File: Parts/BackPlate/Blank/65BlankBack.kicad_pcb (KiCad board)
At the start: 2 copper layers, 172.9 x 20 mm, 3 parts

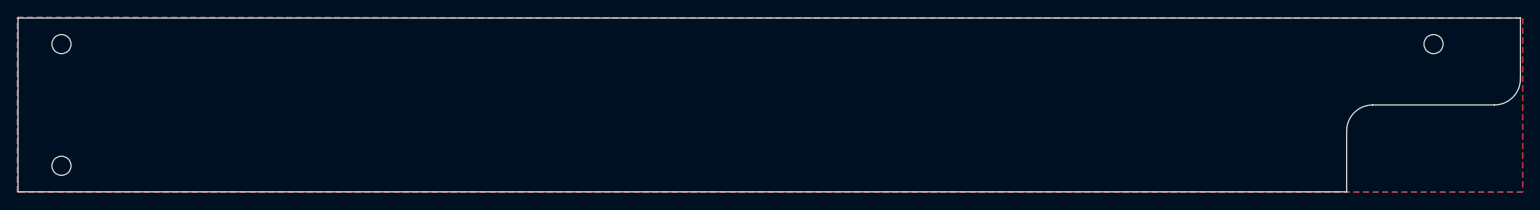
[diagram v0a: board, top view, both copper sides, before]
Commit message: 寸法更新とか
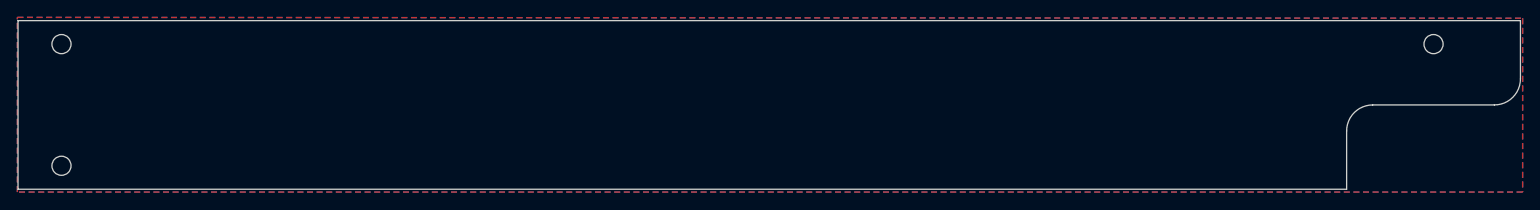
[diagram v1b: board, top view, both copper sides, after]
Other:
- board size 172.9 x 20 mm -> 172.9 x 19.4 mm
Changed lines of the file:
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@@
     (arrow2b (pts (xy 10.925 20) (xy 11.511421 21.126504)))
   )
-  (gr_line (start 14 40) (end 166.875 40) (layer Edge.Cuts) (width 0.1))
-  (gr_line (start 14 20) (end 186.875 20) (layer Edge.Cuts) (width 0.1))
+  (gr_line (start 14 39.7) (end 166.875 39.7) (layer Edge.Cuts) (width 0.1))
+  (gr_line (start 14 20.3) (end 186.875 20.3) (layer Edge.Cuts) (width 0.1))
   (gr_arc (start 183.875 27) (end 183.875 30) (angle -90) (layer Edge.Cuts) (width 0.1))
   (gr_arc (start 169.875 33) (end 169.875 30) (angle -90) (layer Edge.Cuts) (width 0.1))
-  (gr_line (start 186.875 27) (end 186.875 20) (layer Edge.Cuts) (width 0.1))
+  (gr_line (start 186.875 27) (end 186.875 20.3) (layer Edge.Cuts) (width 0.1))
   (gr_line (start 169.875 30) (end 183.875 30) (layer Edge.Cuts) (width 0.1))
-  (gr_line (start 166.875 40) (end 166.875 33) (layer Edge.Cuts) (width 0.1))
-  (gr_line (start 14 20) (end 14 40) (layer Edge.Cuts) (width 0.1))
+  (gr_line (start 166.875 39.7) (end 166.875 33) (layer Edge.Cuts) (width 0.1))
+  (gr_line (start 14 20.3) (end 14 39.7) (layer Edge.Cuts) (width 0.1))
   (zone (net 0) (net_name "") (layer F.Cu) (hatch edge 0.508)
     (connect_pads (clearance 0.508))
